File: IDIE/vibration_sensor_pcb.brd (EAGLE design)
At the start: 61.3 x 43.4 mm, 3 parts, among them IC1 LORA-E5, IC2 STM32L071KBT6

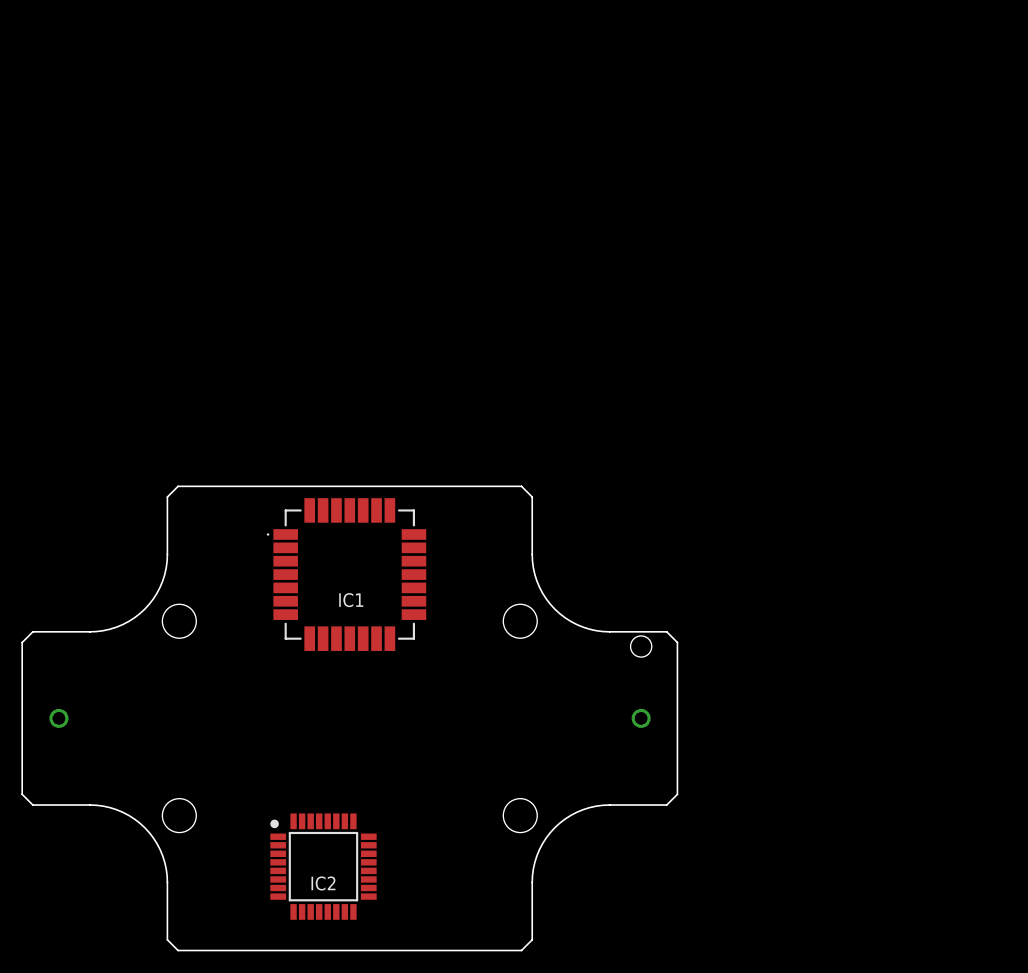
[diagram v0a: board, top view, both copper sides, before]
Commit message: add new design with other modules
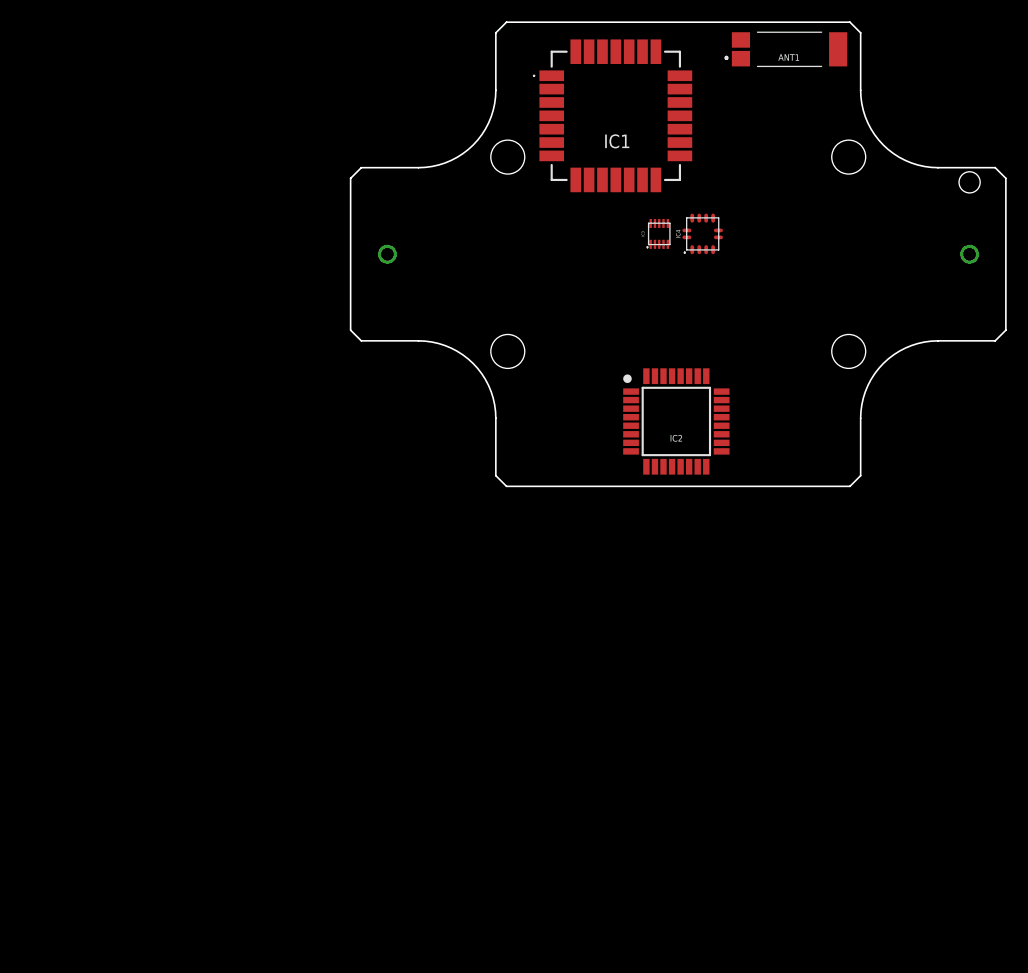
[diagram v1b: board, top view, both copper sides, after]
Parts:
- added ANT1: ANTENNA, SamacSys_Parts:ANTENNA
- added IC3: FXLS8974CFR3, SamacSys_Parts:FXLS8974CFR3
- added IC4: FXLS8971CFR1, SamacSys_Parts:FXLS8971CFR1
- moved H1 53.2 mm to (58.0, 21.7)
- moved IC2 53.2 mm to (30.6, 6.07)
- moved IC1 49.6 mm to (24.9, 34.7)
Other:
- outline, holes or cut-outs redrawn
